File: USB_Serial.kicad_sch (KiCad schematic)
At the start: 2 parts, among them J501 690-005-299-043, U501 MCP2221A-I_SL

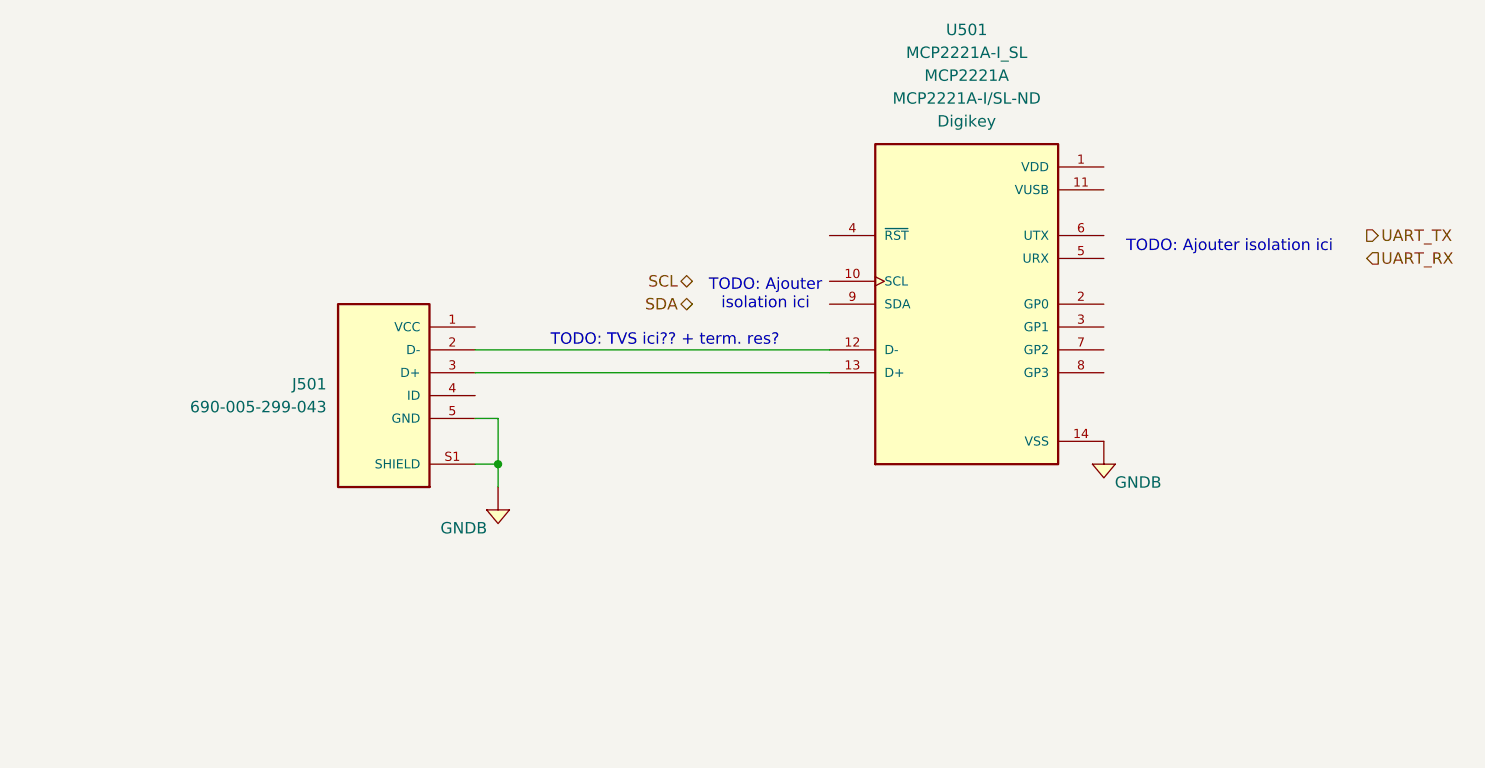
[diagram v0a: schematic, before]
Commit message: update schematique
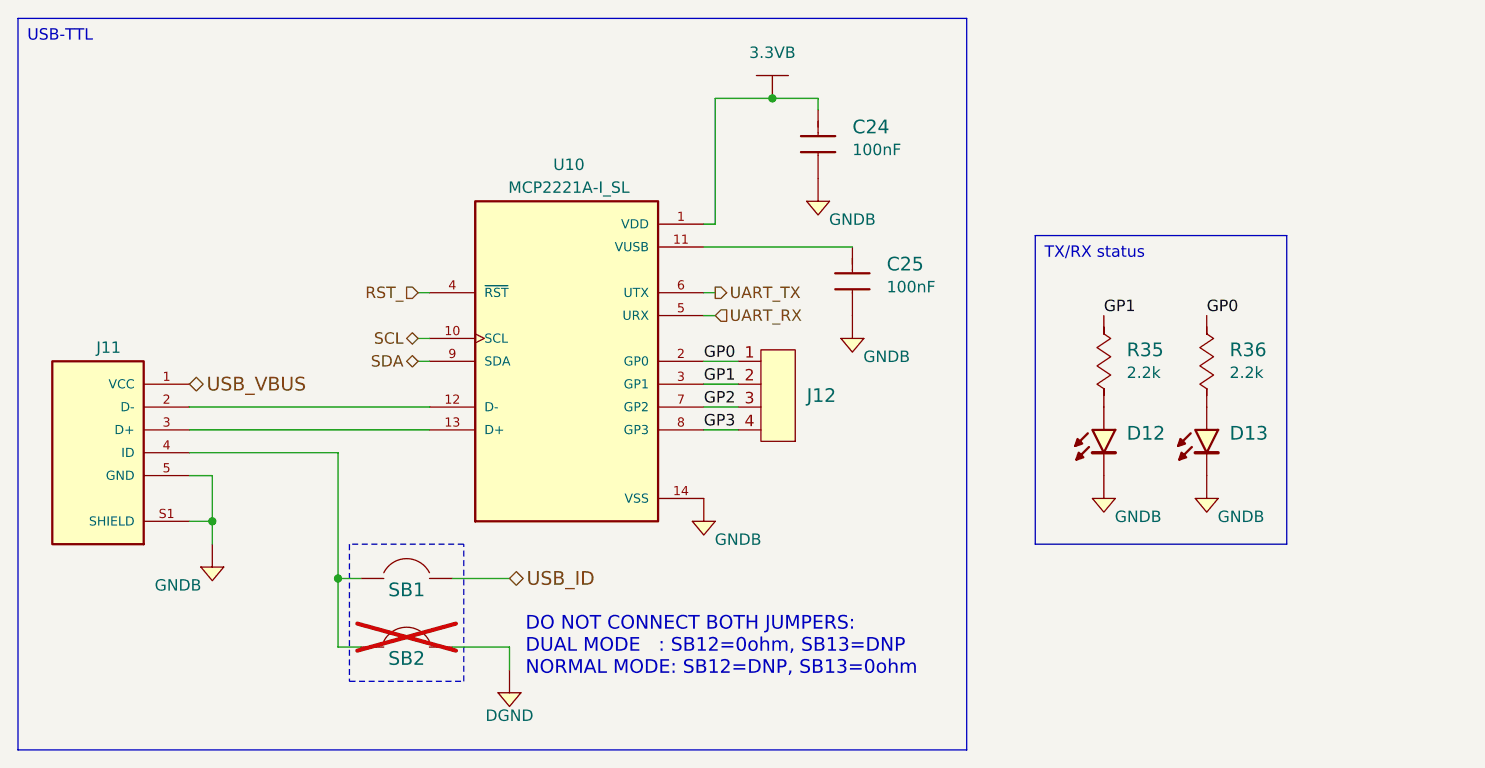
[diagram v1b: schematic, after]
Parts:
- added C24, C25: 885012207098, Capacitors:C0805, symbol Capacitors:885012207098
- added D12: 150080VS75000, Diodes:LED_0805_GREEN, symbol Diodes:150080VS75000
- added D13: 150080YS75000, Diodes:LED_0805_YELLOW, symbol Diodes:150080YS75000
- added J12: Header_Male_Pin_2.54mm_1X4_,_Unshrouded, Connectors:Headers_2.54mm_1X4, symbol Connectors:Header_Male_Pin_2.54mm_1X4_,_Unshrouded
- added R35, R36: RC0805JR-072K2L, Resistors:R0805, symbol Resistors:RC0805JR-072K2L
- added SB1, SB2: Solder_Bridge, Connectors:Solder_bridge_0805, symbol Connectors:Solder_Bridge
- renumbered J501 to J11, U501 to U10
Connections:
- net GNDB: now also C24.1, C25.1, D12.1 (Cathode), D13.1 (Cathode)
- net SCL: now also U10.10 (SCL)
- net SDA: now also U10.9 (SDA)
- net UART_RX: now also U10.5 (URX)
- net UART_TX: now also U10.6 (UTX)
- net USB_VBUS: now reaches J11.1 (VCC)
- net at J11.4 (ID): now also SB1.2, SB2.2
- net 3.3VB: now reaches U10.1 (VDD)
- net 3.3VB: now also C24.2
- net at U10.11 (VUSB): now also C25.2
- net GP0: now reaches U10.2 (GP0)
- net GP0: now also J12.1, R36.2
- net GP1: now reaches U10.3 (GP1)
- net GP1: now also J12.2, R35.2
- net RST_: now reaches U10.4 (~{RST})
- net GP2: now reaches U10.7 (GP2)
- net GP2: now also J12.3
- net GP3: now reaches U10.8 (GP3)
- net GP3: now also J12.4
- new net: D12.2 (Anode), R35.1
- new net: D13.2 (Anode), R36.1
- new net DGND: SB2.1
- new net USB_ID: SB1.1
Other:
- note added: "DO NOT CONNECT BOTH JUMPERS: DUAL MODE : SB12=0ohm, SB13=DNP NORMAL MODE: SB12=DNP, SB13=0ohm"
- note removed: "TODO: Ajouter isolation ici"
- note removed: "TODO: TVS ici?? + term. res?"
- moved on the sheet: J11, U10
